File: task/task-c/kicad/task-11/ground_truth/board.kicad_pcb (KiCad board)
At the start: 2 copper layers, 50 x 55 mm, 4 parts, among them U1 IC

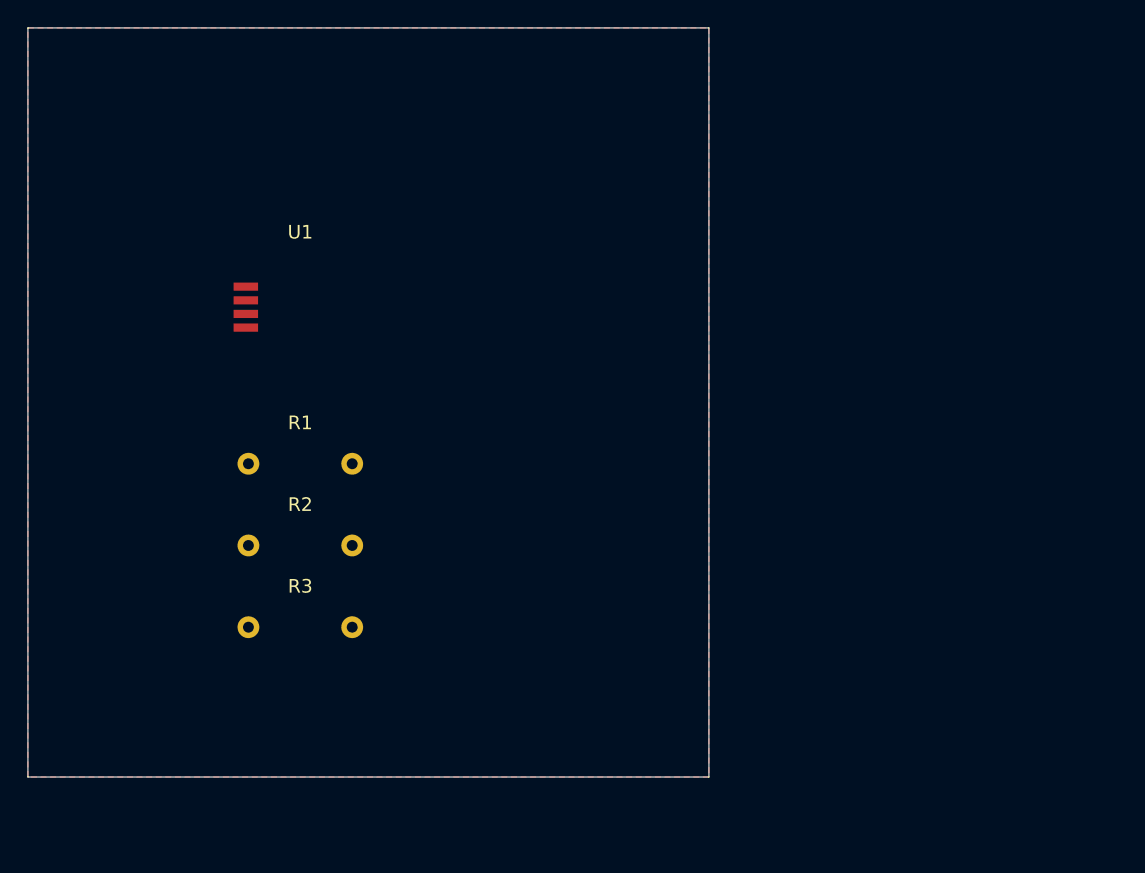
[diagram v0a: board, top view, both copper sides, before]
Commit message: Refine engineering task metadata and instructions
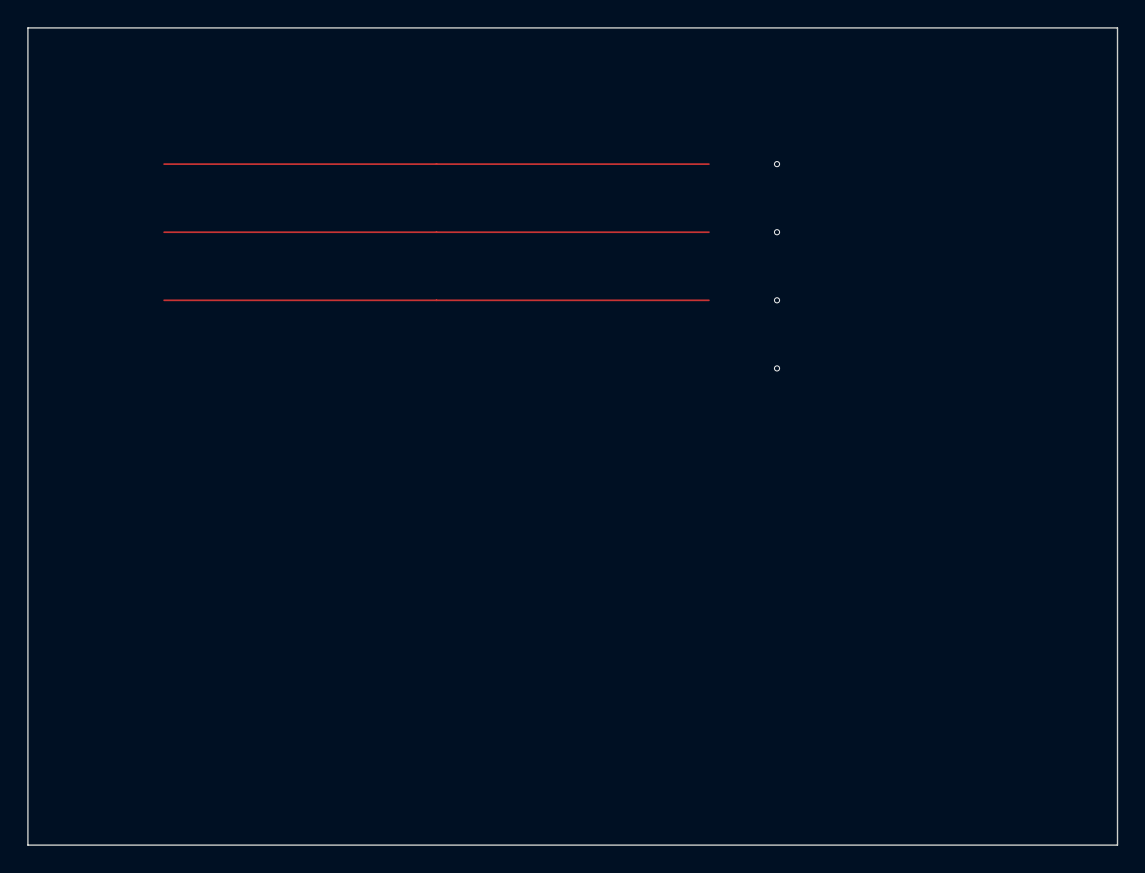
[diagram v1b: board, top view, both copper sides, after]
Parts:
- removed R1, R2: 10k, Resistor_THT:R_Axial_DIN0204_L3.6mm_D1.6mm_P7.62mm_Horizontal
- removed R3: DNP, Resistor_THT:R_Axial_DIN0204_L3.6mm_D1.6mm_P7.62mm_Horizontal
- removed U1: IC, Package_QFP:LQFP-32_7x7mm_P0.8mm
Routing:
- net VCC: track 0.00 -> 40.0 mm, vias 0 -> 1
- net SIG_A: track 0.00 -> 40.0 mm, vias 0 -> 1
- net GND: track 0.00 -> 40.0 mm, vias 0 -> 1
- net SIG_B: vias 0 -> 1
- removed copper zone on F.Cu, net GND
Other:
- board size 50 x 55 mm -> 80 x 60 mm
- rule pad_to_mask_clearance: 0.051 -> 0.1
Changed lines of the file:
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@@
   (version 20240108)
   (generator "pcbnew")
-  (general (thickness 1.6) (legacy_teardrops no))
+  (generator_version "9.0")
+  (general
+    (thickness 1.6)
+    (legacy_teardrops no)
+  )
   (paper "A4")
   (layers
     (0 "F.Cu" signal)
     (31 "B.Cu" signal)
-    (36 "B.SilkS" user "B.Silkscreen")
-    (37 "F.SilkS" user "F.Silkscreen")
-    (49 "Edge.Cuts" user)
+    (44 "Edge.Cuts" user)
   )
-  (setup (pad_to_mask_clearance 0.051))
+  (setup
+    (pad_to_mask_clearance 0.1)
+    (allow_soldermask_bridges_in_footprints no)
+  )
   (net 0 "")
-  (net 1 "GND")
-  (net 2 "VCC")
+  (net 1 "VCC")
+  (net 2 "GND")
   (net 3 "SIG_A")
   (net 4 "SIG_B")
-  (net 5 "DNC_NET")
-  (footprint "Package_QFP:LQFP-32_7x7mm_P0.8mm"
-    (layer "F.Cu")
-    (at 20 20)
-    (property "Reference" "U1" (at 0 -5) (layer "F.SilkS") (effects (font (size 1 1) (thickness 0.15))))
-    (property "Value" "IC" (at 0 5) (layer "F.Fab") (effects (font (size 1 1) (thickness 0.15))))
-    (pad "1" smd rect (at -4 -1) (size 1.8 0.6) (layers "F.Cu" "F.Paste" "F.Mask") (net 2 "VCC") (zone_connect 2))
-    (pad "2" smd rect (at -4 0) (size 1.8 0.6) (layers "F.Cu" "F.Paste" "F.Mask") (net 2 "VCC") (zone_connect 2))
-    (pad "3" smd rect (at -4 1) (size 1.8 0.6) (layers "F.Cu" "F.Paste" "F.Mask") (net 3 "SIG_A"))
-    (pad "4" smd rect (at -4 2) (size 1.8 0.6) (layers "F.Cu" "F.Paste" "F.Mask") (net 1 "GND") (zone_connect 2))
-  )
-  (footprint "Resistor_THT:R_Axial_DIN0204_L3.6mm_D1.6mm_P7.62mm_Horizontal"
-    (layer "F.Cu")
-    (at 20 32)
-    (property "Reference" "R1" (at 0 -3) (layer "F.SilkS") (effects (font (size 1 1) (thickness 0.15))))
-    (property "Value" "10k" (at 0 3) (layer "F.Fab") (effects (font (size 1 1) (thickness 0.15))))
-    (pad "1" thru_hole circle (at -3.81 0) (size 1.6 1.6) (drill 0.8) (layers "*.Cu" "*.Mask") (net 3 "SIG_A") (zone_connect 1) (thermal_width 0.4))
-    (pad "2" thru_hole circle (at 3.81 0) (size 1.6 1.6) (drill 0.8) (layers "*.Cu" "*.Mask") (net 1 "GND") (zone_connect 1) (thermal_width 0.4))
-  )
-  (footprint "Resistor_THT:R_Axial_DIN0204_L3.6mm_D1.6mm_P7.62mm_Horizontal"
-    (layer "F.Cu")
-    (at 20 38)
-    (property "Reference" "R2" (at 0 -3) (layer "F.SilkS") (effects (font (size 1 1) (thickness 0.15))))
-    (property "Value" "10k" (at 0 3) (layer "F.Fab") (effects (font (size 1 1) (thickness 0.15))))
-    (pad "1" thru_hole circle (at -3.81 0) (size 1.6 1.6) (drill 0.8) (layers "*.Cu" "*.Mask") (net 4 "SIG_B") (zone_connect 1) (thermal_width 0.4))
-    (pad "2" thru_hole circle (at 3.81 0) (size 1.6 1.6) (drill 0.8) (layers "*.Cu" "*.Mask") (net 1 "GND") (zone_connect 1) (thermal_width 0.4))
-  )
-  (footprint "Resistor_THT:R_Axial_DIN0204_L3.6mm_D1.6mm_P7.62mm_Horizontal"
-    (layer "F.Cu")
-    (at 20 44)
-    (property "Reference" "R3" (at 0 -3) (layer "F.SilkS") (effects (font (size 1 1) (thickness 0.15))))
-    (property "Value" "DNP" (at 0 3) (layer "F.Fab") (effects (font (size 1 1) (thickness 0.15))))
-    (pad "1" thru_hole circle (at -3.81 0) (size 1.6 1.6) (drill 0.8) (layers "*.Cu" "*.Mask") (net 5 "DNC_NET") (zone_connect 0))
-    (pad "2" thru_hole circle (at 3.81 0) (size 1.6 1.6) (drill 0.8) (layers "*.Cu" "*.Mask") (net 5 "DNC_NET") (zone_connect 0))
-  )
-  (zone
-    (net 1)
-    (net_name "GND")
-    (layer "F.Cu")
-    (name "GND_TOP")
-    (hatch edge 0.508)
-    (connect_pads (clearance 0.5))
-    (min_thickness 0.25)
-    (fill yes (thermal_gap 0.5) (thermal_bridge_width 0.3))
-    (polygon (pts (xy 0 0) (xy 50 0) (xy 50 55) (xy 0 55)))
-  )
-  (gr_rect (start 0 0) (end 50 55) (layer "Edge.Cuts") (width 0.05))
+  (net 5 "SIG_C")
+  (segment (start 10 10) (end 30 10) (width 0.127) (layer "F.Cu") (net 1))
+  (segment (start 30 10) (end 50 10) (width 0.127) (layer "F.Cu") (net 1))
+  (segment (start 10 15) (end 30 15) (width 0.127) (layer "F.Cu") (net 2))
+  (segment (start 30 15) (end 50 15) (width 0.127) (layer "F.Cu") (net 2))
+  (segment (start 10 20) (end 30 20) (width 0.127) (layer "F.Cu") (net 3))
+  (segment (start 30 20) (end 50 20) (width 0.127) (layer "F.Cu") (net 3))
+  (via (at 55 10) (size 0.452) (drill 0.30) (layers "F.Cu" "B.Cu") (net 1))
+  (via (at 55 15) (size 0.452) (drill 0.30) (layers "F.Cu" "B.Cu") (net 2))
+  (via (at 55 20) (size 0.452) (drill 0.30) (layers "F.Cu" "B.Cu") (net 3))
+  (via (at 55 25) (size 0.452) (drill 0.30) (layers "F.Cu" "B.Cu") (net 4))
+  (gr_rect (start 0 0) (end 80 60) (layer "Edge.Cuts") (width 0.1))
 )
